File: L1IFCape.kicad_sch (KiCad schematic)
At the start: 85 parts, among them J1 RF_Shield_One_Piece, J2 SMA, J3 MMCX, P8 BeagleBone_Black_Header, P9 BeagleBone_Black_Header, U1 24CS256, U2 MAX2769BETI+T, U3 MAX31343ETAY+T, U4 TPS717285DCK, U5 TPS717285DCK, X1 SIT5156, X2 QPQ1060

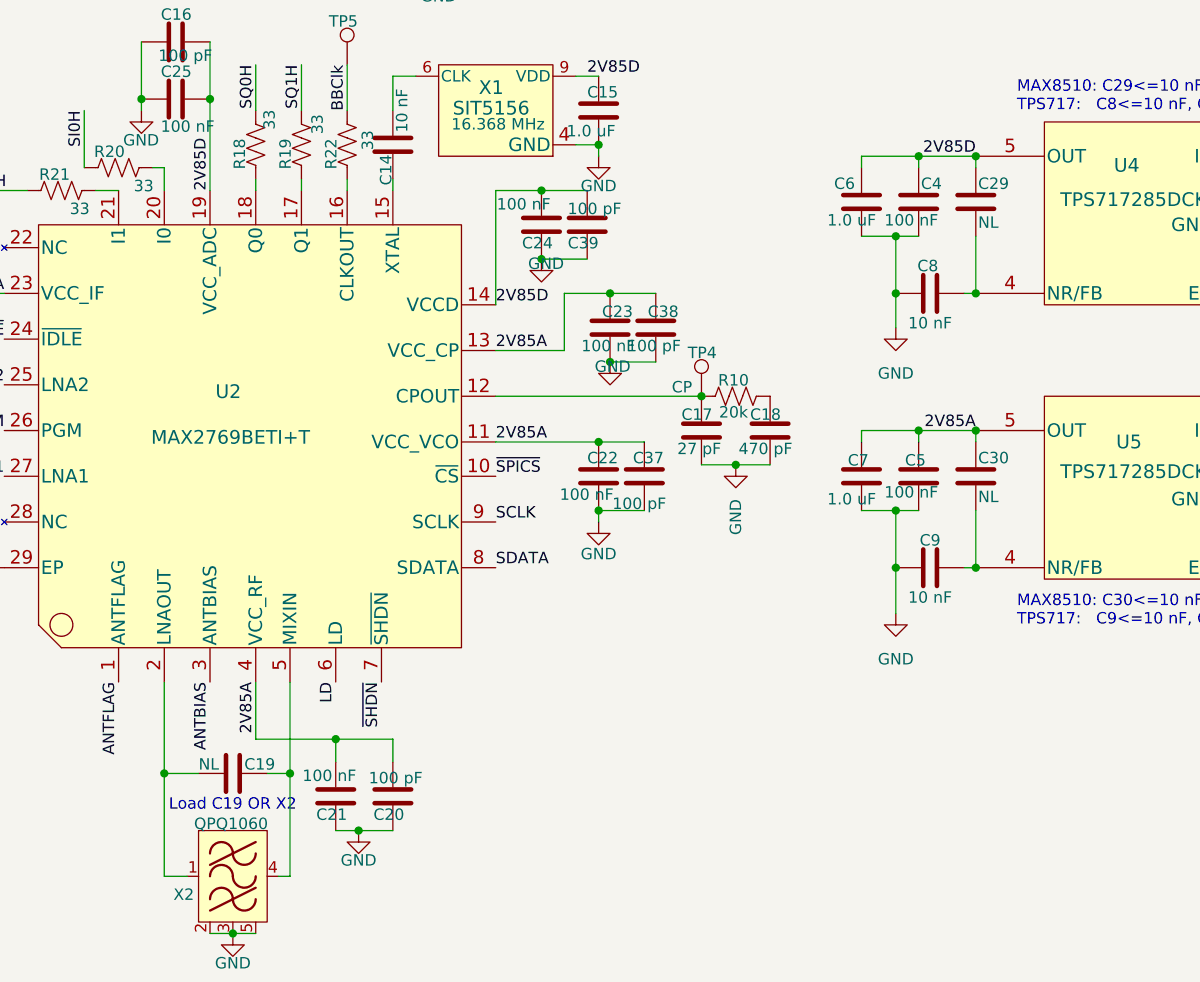
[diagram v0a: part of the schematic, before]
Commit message: Creating BOM
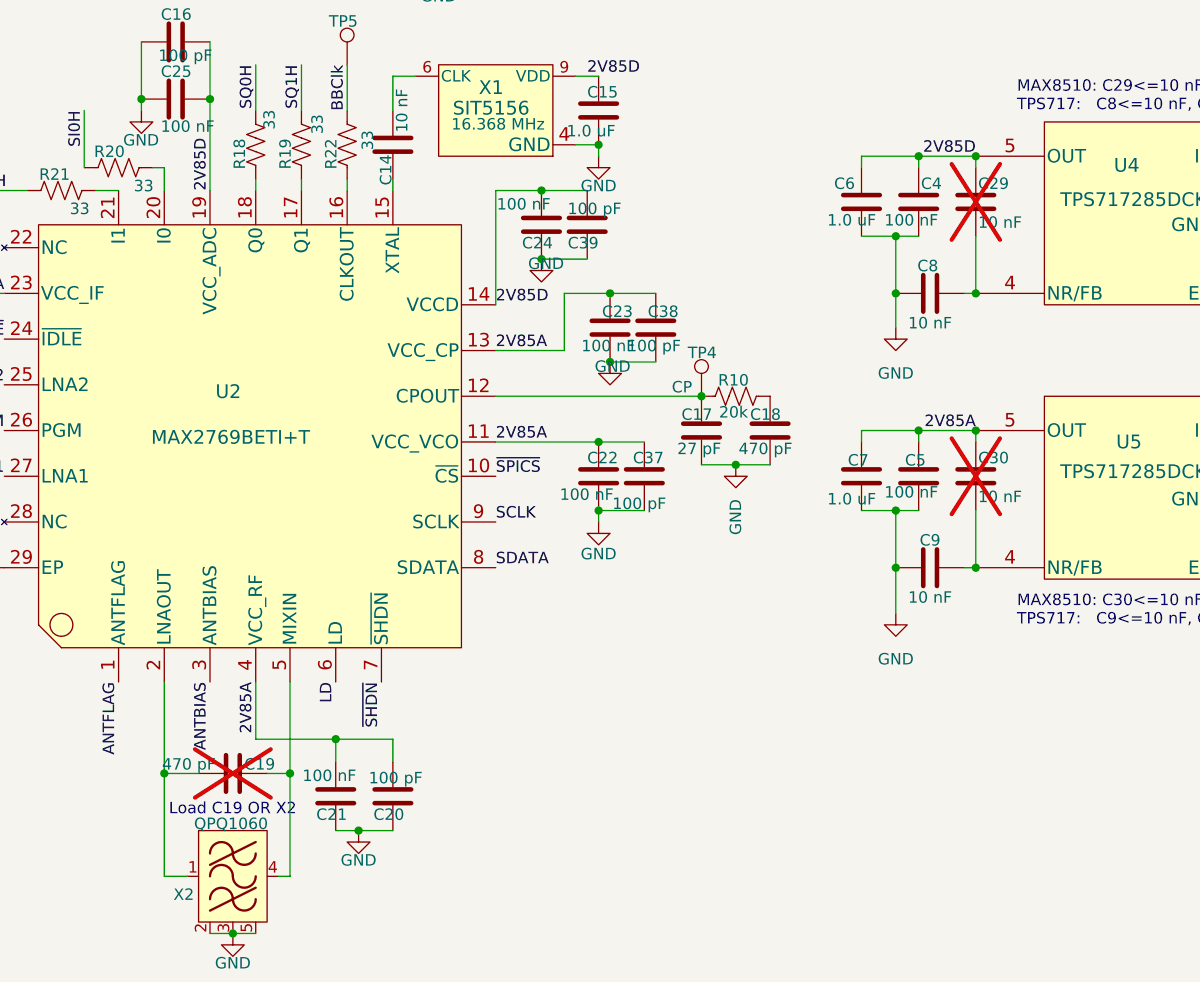
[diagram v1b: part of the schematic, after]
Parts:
- C10, C11, C18: VPN (none) -> 490-GCM1885C2A471FA16DCT-ND
- C13, C21, C22, C23, C24, C25, C26, C4, C5: VPN (none) -> 399-6856-1-ND
- C14, C8, C9: VPN (none) -> 399-C0603C103F3GECAUTOCT-ND
- C15, C2, C27, C28, C3, C35, C6, C7: VPN (none) -> 490-5241-1-ND
- C17: VPN (none) -> 399-C0603C270F3HACAUTOCT-ND
- C19: value NL -> 470 pF; now not fitted
- C29, C30: value NL -> 10 nF; now not fitted
- C31, C33: VPN (none) -> 399-15708-1-ND
- C32, C34: VPN (none) -> 399-C0805C104K8RACTUCT-ND
- FB1, FB2: VPN (none) -> 490-14399-1-ND
- J1: VPN (none) -> 903-1008-1-ND
- J2: VPN (none) -> ARF1206-ND
- J3: VPN (none) -> ARF1904-ND
- P8, P9: VPN (none) -> 612-SSQ-123-23-G-D-ND
- R1, R3, R4, R6: MFR (none) -> Panasonic; MPN (none) -> ERJ-3GEY0R00V; VPN (none) -> P0.0GCT-ND; Vendor (none) -> DigiKey; Vendor PN (none) -> P0.0GCT-ND
- R10: MFR (none) -> Panasonic; VPN (none) -> P20.0KHCT-ND
- R11, R12, R18, R19, R20, R21, R22, R7, R8, R9: MFR (none) -> Panasonic; MPN (none) -> ERJ-3EKF33R0V; VPN (none) -> P33.0HCT-ND; Vendor (none) -> Digikey
- R17: VPN (none) -> P10.0KHCT-ND
- R2, R5: DNP (none) -> 0; MFR (none) -> Panasonic; MPN (none) -> ERJ-3GEY0R00V; VPN (none) -> P0.0GCT-ND; Vendor (none) -> DigiKey; Vendor PN (none) -> P0.0GCT-ND
- TP5: value ~{SHDN} -> BBClk
